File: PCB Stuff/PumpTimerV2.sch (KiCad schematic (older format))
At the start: 32 parts, among them J1 1935161, J2 282856-2, J3 282856-2, J4 Conn_02x20_Odd_Even, J6 B4B-PH-SM4-TBT(LF)(SN), K1 ADW1205HLW, K2 ADW1205HLW, Q1 DMN67D7L, Q2 DMN67D7L, SW1 TL3305AF160QG, U1 RX8900UA

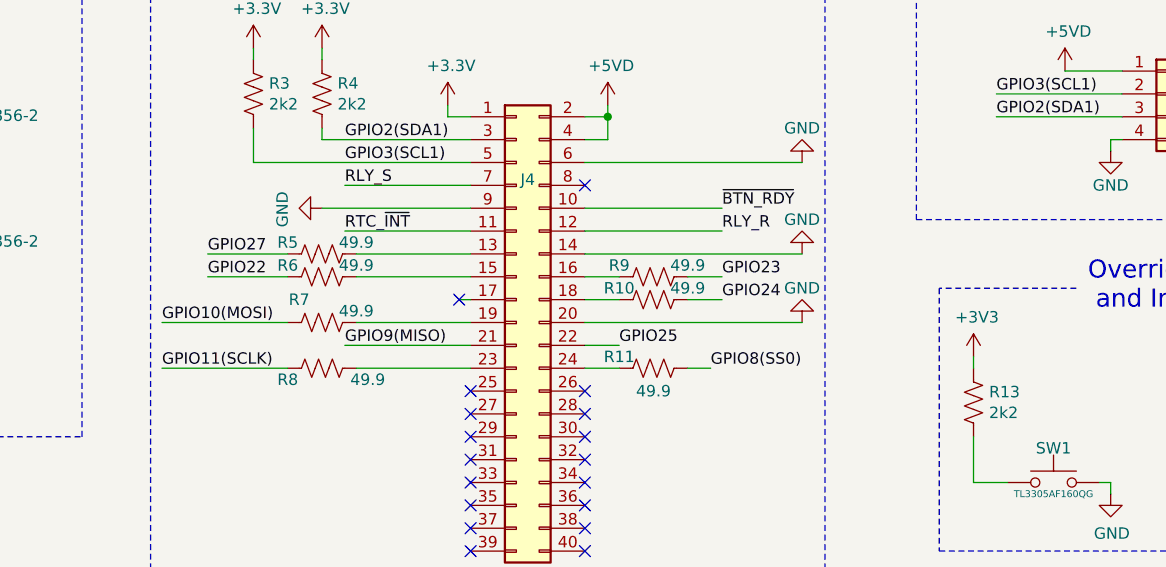
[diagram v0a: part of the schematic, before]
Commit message: Routing and placement
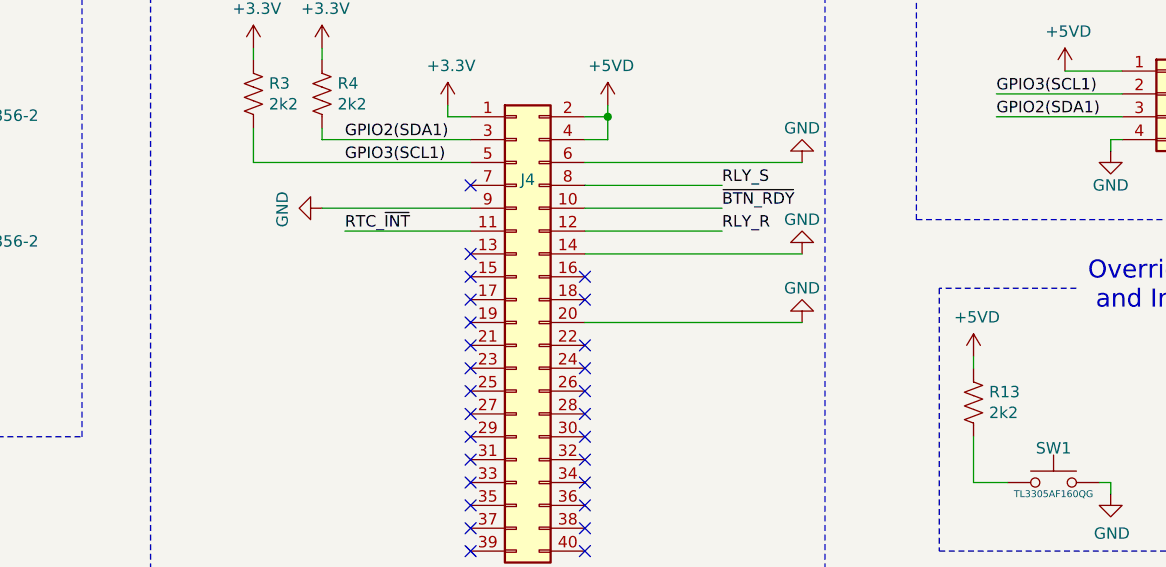
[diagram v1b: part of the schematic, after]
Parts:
- removed R10, R11, R5, R6, R7, R8, R9: 49.9, Resistor_SMD:R_0603_1608Metric_Pad0.98x0.95mm_HandSolder, symbol Device:R_US
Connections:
- net +3V3: no longer R13.1
- net +5VD: now also R13.1
- net RLY_S: now also J4.8 (Pin_8); no longer J4.7 (Pin_7)
- net GPIO25: no longer names the net of J4.22 (Pin_22)
- net GPIO9(MISO): no longer names the net of J4.21 (Pin_21)
- no-connect marks 19 -> 28
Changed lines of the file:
@@
 Text Label 6150 2350 0    50   ~ 0
 RTC_~INT~
-Text Label 5550 2450 0    50   ~ 0
-GPIO27
-Text Label 5550 2550 0    50   ~ 0
-GPIO22
-NoConn ~ 6650 2650
-Wire Wire Line
-	6700 2650 6650 2650
-Text Label 5350 2750 0    50   ~ 0
-GPIO10(MOSI)
-Text Label 5350 2950 0    50   ~ 0
-GPIO11(SCLK)
 Wire Wire Line
 	6050 2250 6700 2250
 Wire Wire Line
 	6700 2350 6150 2350
-Wire Wire Line
-	6700 2850 6150 2850
 $Comp
 L power:GND #PWR023
@@
 	-1   0    0    1
 $EndComp
-Text Label 7800 2550 0    50   ~ 0
-GPIO23
-Text Label 7800 2650 0    50   ~ 0
-GPIO24
 $Comp
 L power:GND #PWR024
@@
 	-1   0    0    1
 $EndComp
-Text Label 7350 2850 0    50   ~ 0
-GPIO25
-Text Label 7750 2950 0    50   ~ 0
-GPIO8(SS0)
-Wire Wire Line
-	7200 2850 7350 2850
-Wire Wire Line
-	7350 2950 7200 2950
-Wire Wire Line
-	7200 2650 7350 2650
-Wire Wire Line
-	7200 2550 7350 2550
 $Comp
 L Diode:Generic_Diode D2
@@
 $EndComp
 $Comp
-L Device:R_US R7
-U 1 1 607C006A
-P 6050 2750
-F 0 "R7" V 5950 2650 50  0000 C CNN
-F 1 "49.9" V 6000 2900 50  0000 C CNN
-F 2 "Resistor_SMD:R_0603_1608Metric_Pad0.98x0.95mm_HandSolder" V 6090 2740 50  0001 C CNN
-F 3 "ERJ-3EKF49R9V" H 6050 2750 50  0001 C CNN
-	1    6050 2750
-	0    1    1    0
-$EndComp
-Text Label 6150 2850 0    50   ~ 0
-GPIO9(MISO)
-Wire Wire Line
-	5900 2950 5350 2950
-Wire Wire Line
-	5350 2750 5900 2750
-Wire Wire Line
-	6200 2750 6700 2750
-Wire Wire Line
-	6700 2950 6200 2950
-$Comp
-L Device:R_US R11
-U 1 1 607CC497
-P 7500 2950
-F 0 "R11" V 7450 2800 50  0000 C CNN
-F 1 "49.9" V 7600 2950 50  0000 C CNN
-F 2 "Resistor_SMD:R_0603_1608Metric_Pad0.98x0.95mm_HandSolder" V 7540 2940 50  0001 C CNN
-F 3 "ERJ-3EKF49R9V" H 7500 2950 50  0001 C CNN
-	1    7500 2950
-	0    1    1    0
-$EndComp
-Wire Wire Line
-	7650 2950 7750 2950
-$Comp
-L Device:R_US R8
-U 1 1 607D7BAE
-P 6050 2950
-F 0 "R8" V 6100 2800 50  0000 C CNN
-F 1 "49.9" V 6100 3150 50  0000 C CNN
-F 2 "Resistor_SMD:R_0603_1608Metric_Pad0.98x0.95mm_HandSolder" V 6090 2940 50  0001 C CNN
-F 3 "ERJ-3EKF49R9V" H 6050 2950 50  0001 C CNN
-	1    6050 2950
-	0    1    1    0
-$EndComp
-$Comp
 L Device:C C1
 U 1 1 607DE07A
@@
 	-1   0    0    1
 $EndComp
-$Comp
-L Device:R_US R9
-U 1 1 607F57A6
-P 7500 2550
-F 0 "R9" V 7450 2400 50  0000 C CNN
-F 1 "49.9" V 7450 2700 50  0000 C CNN
-F 2 "Resistor_SMD:R_0603_1608Metric_Pad0.98x0.95mm_HandSolder" V 7540 2540 50  0001 C CNN
-F 3 "ERJ-3EKF49R9V" H 7500 2550 50  0001 C CNN
-	1    7500 2550
-	0    1    1    0
-$EndComp
-$Comp
-L Device:R_US R10
-U 1 1 607F6412
-P 7500 2650
-F 0 "R10" V 7450 2500 50  0000 C CNN
-F 1 "49.9" V 7450 2800 50  0000 C CNN
-F 2 "Resistor_SMD:R_0603_1608Metric_Pad0.98x0.95mm_HandSolder" V 7540 2640 50  0001 C CNN
-F 3 "ERJ-3EKF49R9V" H 7500 2650 50  0001 C CNN
-	1    7500 2650
-	0    1    1    0
-$EndComp
-Wire Wire Line
-	7650 2650 7800 2650
-Wire Wire Line
-	7650 2550 7800 2550
 Wire Wire Line
 	7200 2450 8150 2450
@@
 	9000 1750 9550 1750
 $Comp
-L Device:R_US R5
-U 1 1 60879D01
-P 6050 2450
-F 0 "R5" V 6000 2300 50  0000 C CNN
-F 1 "49.9" V 6000 2600 50  0000 C CNN
-F 2 "Resistor_SMD:R_0603_1608Metric_Pad0.98x0.95mm_HandSolder" V 6090 2440 50  0001 C CNN
-F 3 "ERJ-3EKF49R9V" H 6050 2450 50  0001 C CNN
-	1    6050 2450
-	0    1    1    0
-$EndComp
-$Comp
-L Device:R_US R6
-U 1 1 6087A462
-P 6050 2550
-F 0 "R6" V 6000 2400 50  0000 C CNN
-F 1 "49.9" V 6000 2700 50  0000 C CNN
-F 2 "Resistor_SMD:R_0603_1608Metric_Pad0.98x0.95mm_HandSolder" V 6090 2540 50  0001 C CNN
-F 3 "ERJ-3EKF49R9V" H 6050 2550 50  0001 C CNN
-	1    6050 2550
-	0    1    1    0
-$EndComp
-Wire Wire Line
-	5550 2550 5900 2550
-Wire Wire Line
-	5900 2450 5550 2450
-Wire Wire Line
-	6200 2450 6700 2450
-Wire Wire Line
-	6700 2550 6200 2550
-$Comp
 L power:GND #PWR035
 U 1 1 6088F768
@@
 	1    0    0    -1
 $EndComp
-NoConn ~ 7200 2150
 Text Notes 9300 1200 0    79   ~ 0
 I2C Expansion Port\n   (just in case)
@@
 Wire Wire Line
 	2000 6750 2300 6750
-Text Label 6150 2150 0    50   ~ 0
+Text Label 7800 2150 0    50   ~ 0
 RLY_S
-Wire Wire Line
-	6150 2150 6700 2150
-Text Label 7800 2350 0    50   ~ 0
-RLY_R
-Wire Wire Line
-	7800 2350 7200 2350
 Text Label 2000 6750 0    50   ~ 0
 RLY_S
@@
 F 3 "" H 10800 3300 50  0001 C CNN
 	1    10800 3300
-	1    0    0    -1
-$EndComp
-$Comp
-L power:+3V3 #PWR0103
-U 1 1 60797B23
-P 8900 2900
-F 0 "#PWR0103" H 8900 2750 50  0001 C CNN
-F 1 "+3V3" H 8915 3073 50  0000 C CNN
-F 2 "" H 8900 2900 50  0001 C CNN
-F 3 "" H 8900 2900 50  0001 C CNN
-	1    8900 2900
 	1    0    0    -1
 $EndComp
@@
 NoConn ~ 7200 3050
 NoConn ~ 7200 3450
+$Comp
+L power:+5VD #PWR0103
+U 1 1 607FB41A
+P 8900 2900
+F 0 "#PWR0103" H 8900 2750 50  0001 C CNN
+F 1 "+5VD" H 8915 3073 50  0000 C CNN
+F 2 "" H 8900 2900 50  0001 C CNN
+F 3 "" H 8900 2900 50  0001 C CNN
+	1    8900 2900
+	1    0    0    -1
+$EndComp
+Wire Wire Line
+	7800 2350 7200 2350
+Text Label 7800 2350 0    50   ~ 0
+RLY_R
+Wire Wire Line
+	7200 2150 7800 2150
+NoConn ~ 6700 2150
+NoConn ~ 7200 2550
+NoConn ~ 7200 2650
+NoConn ~ 7200 2950
+NoConn ~ 7200 2850
+NoConn ~ 6700 2450
+NoConn ~ 6700 2550
+NoConn ~ 6700 2750
+NoConn ~ 6700 2850
+NoConn ~ 6700 2950
+NoConn ~ 6700 2650
 $EndSCHEMATC
